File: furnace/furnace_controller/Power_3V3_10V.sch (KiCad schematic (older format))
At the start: 30 parts, among them Q2 BC847, Q3 IRLML6402, Q4 IRLML2402, U2 AMS1117-3.3

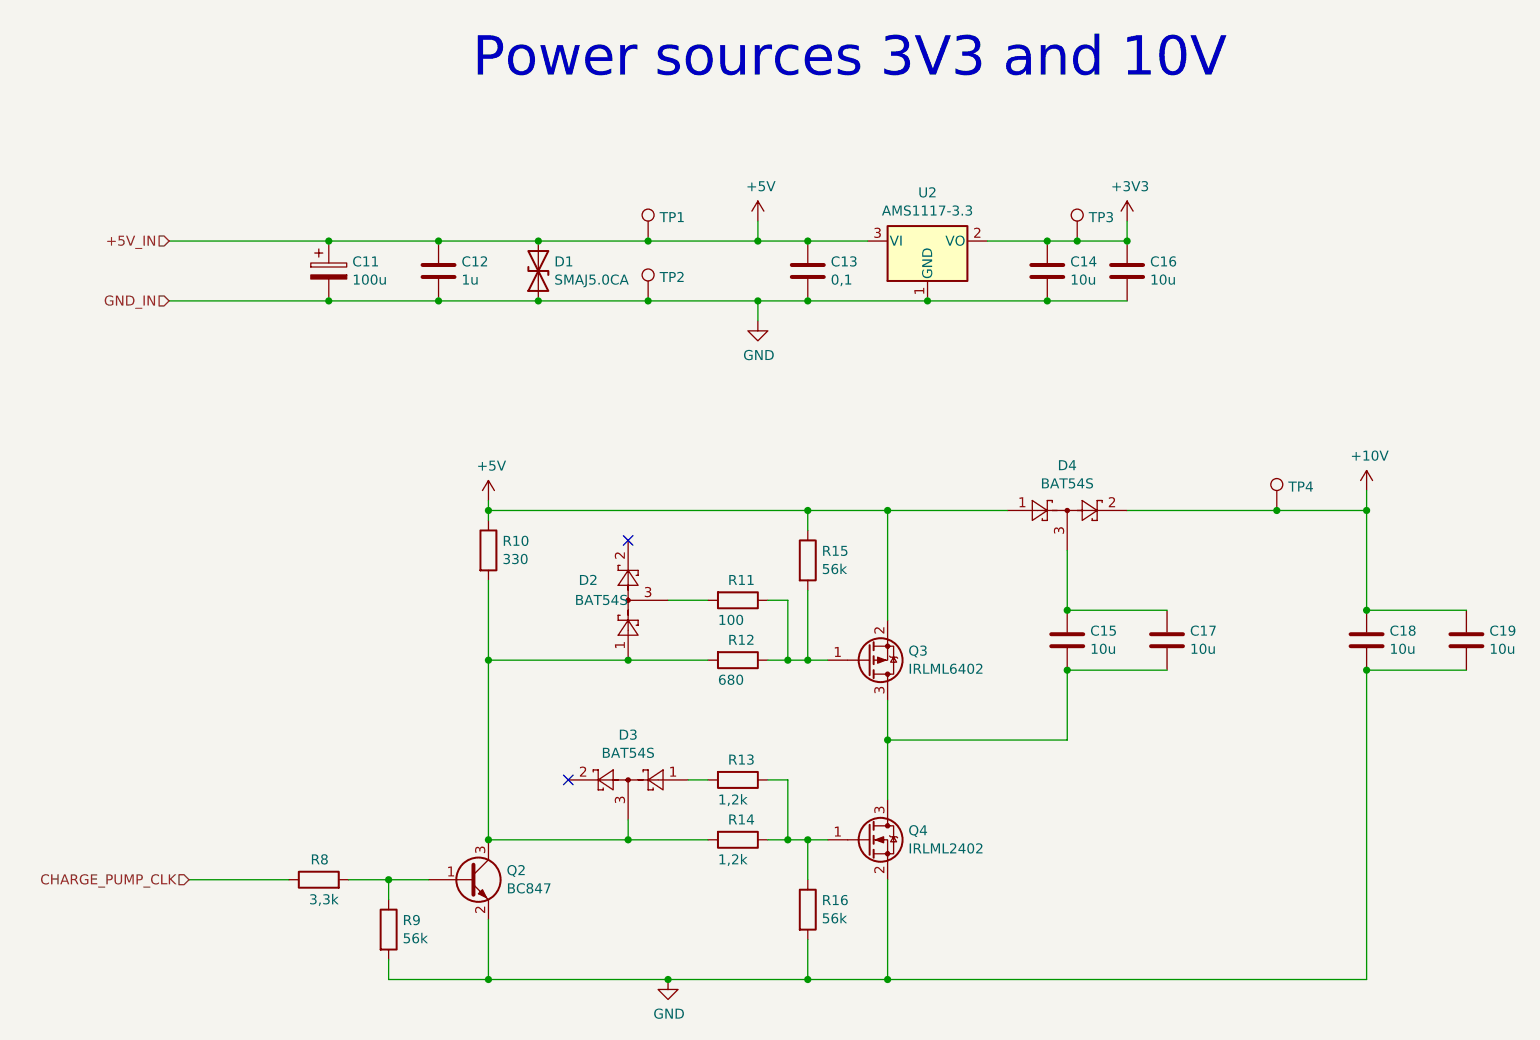
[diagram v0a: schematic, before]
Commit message: Add files via upload
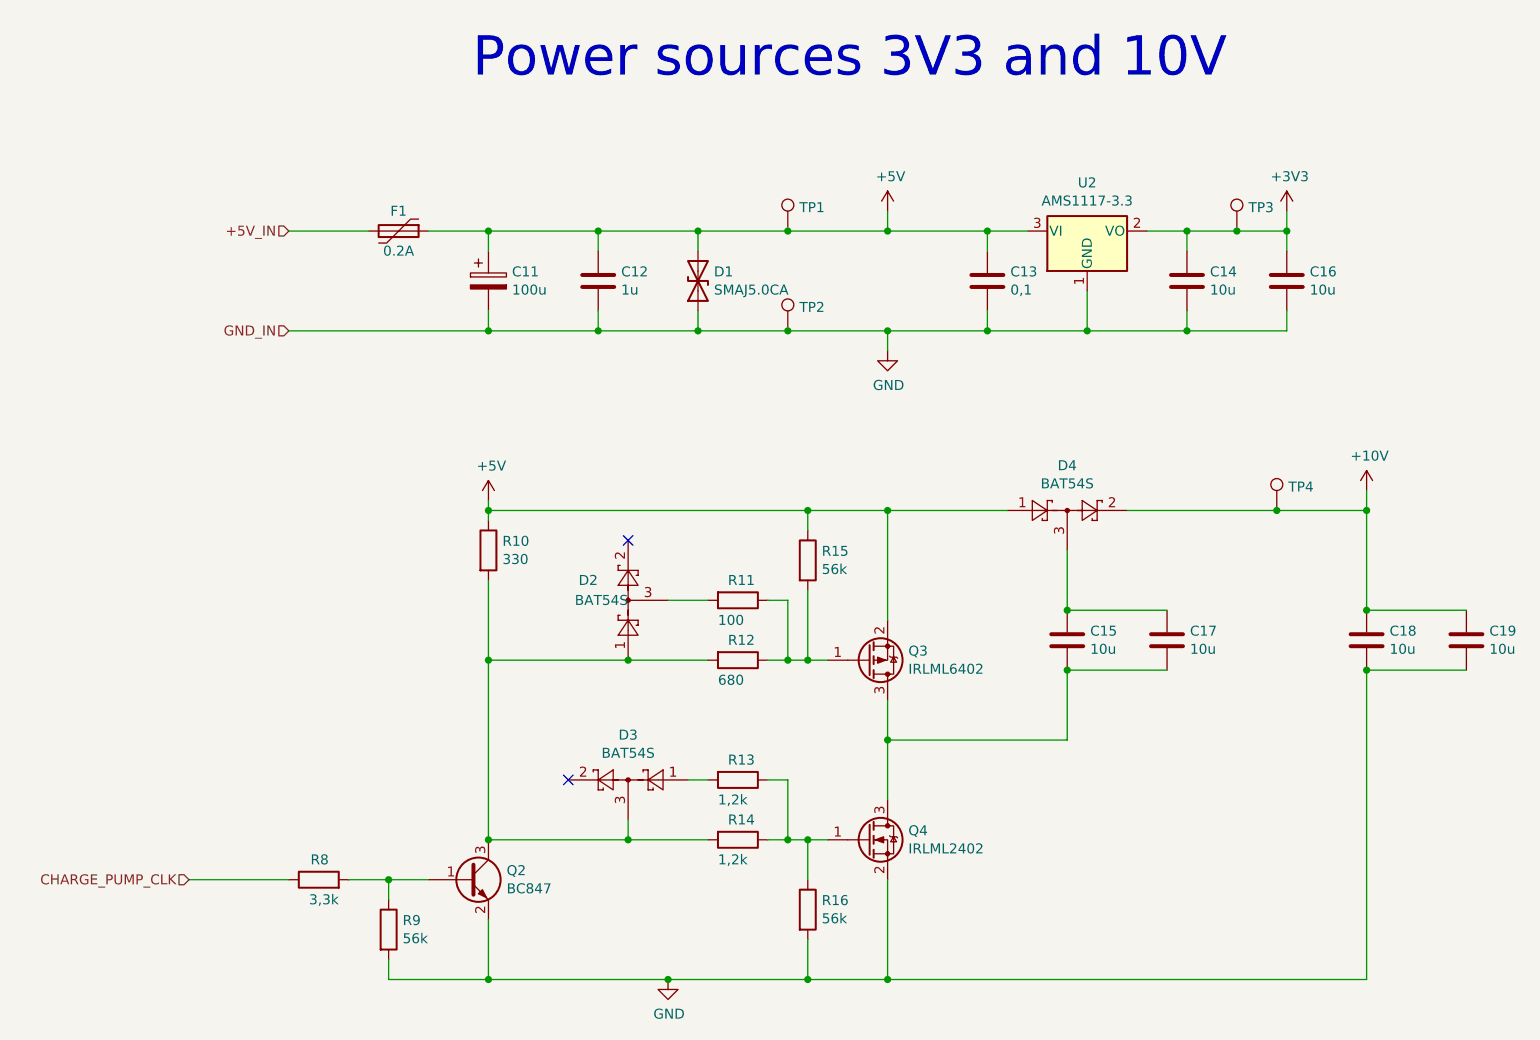
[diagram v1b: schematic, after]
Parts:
- added F1: 0.2A, symbol Device:Polyfuse
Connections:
- net +5V: now also F1.1
- new net +5V_IN: F1.2
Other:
- moved on the sheet: C11, C12, C13, C14, C16, D1, TP1, TP2, TP3, U2
